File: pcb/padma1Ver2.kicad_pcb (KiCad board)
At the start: 2 copper layers, 33 x 68.6 mm, 15 parts, among them SW1 SPST

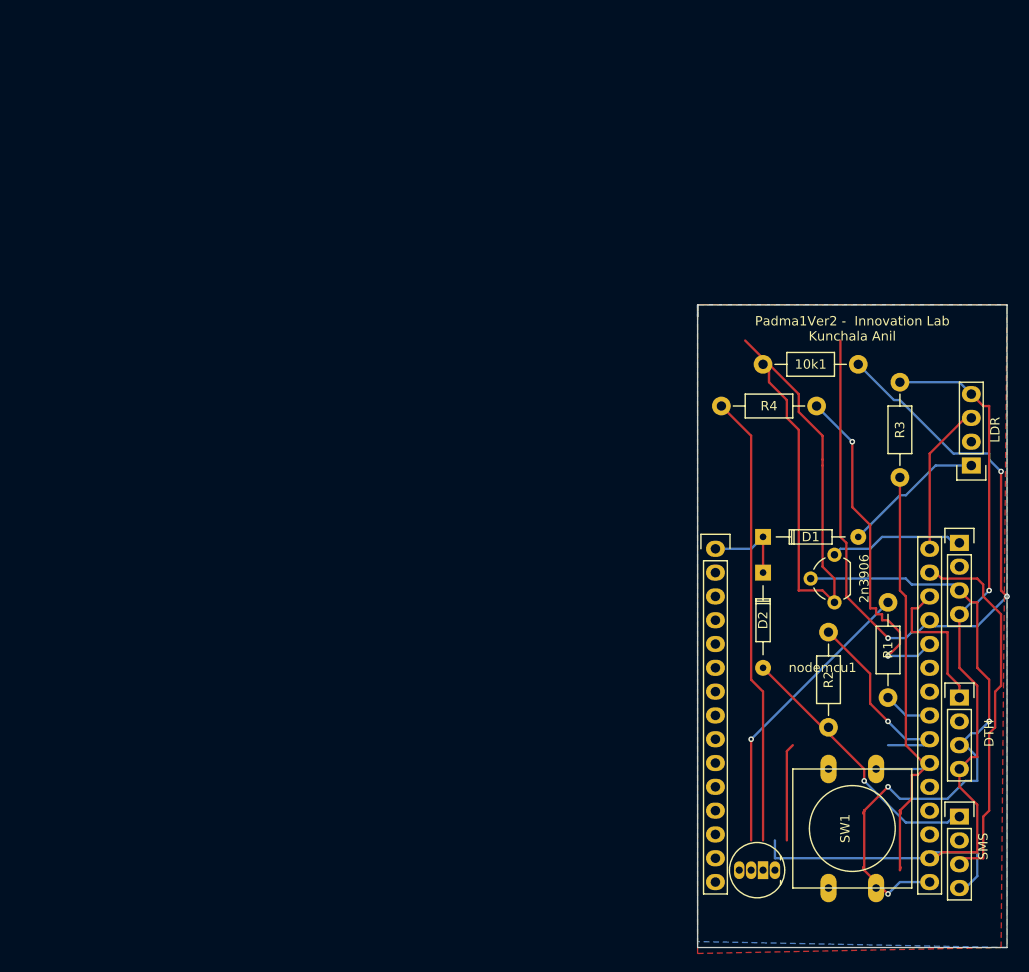
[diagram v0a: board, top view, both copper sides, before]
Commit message: pcb Without Any Errors
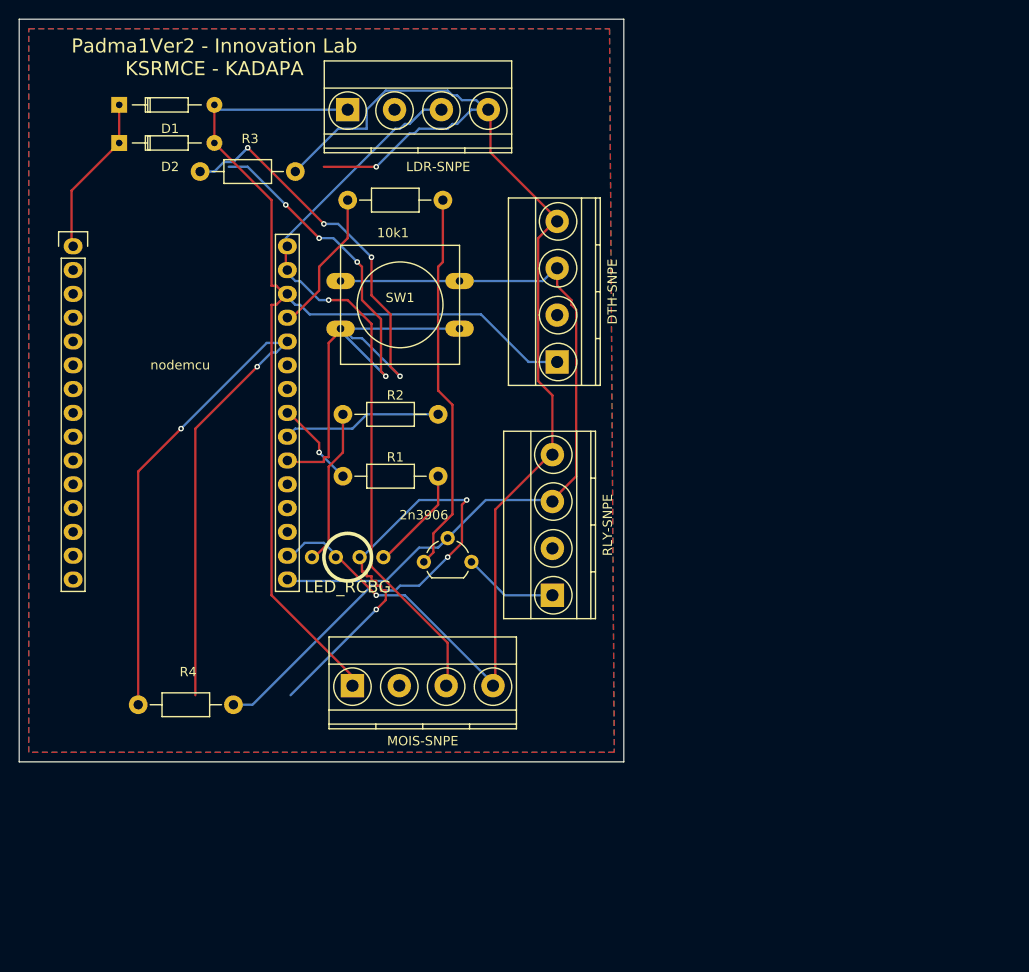
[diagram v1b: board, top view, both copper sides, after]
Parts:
- removed DTH, LDR, SMS: CONN_01X04, Pin_Headers:Pin_Header_Straight_1x04
- removed Grovr1: RLY, Pin_Headers:Pin_Header_Straight_1x04
- removed nodemcu1: nodemcu, nodemcu:NodeMCU_Amica_R2
- added DTH-SNPE: CONN_01X04, Terminal_Blocks:TerminalBlock_Pheonix_MKDS1.5-4pol, F.Cu at (128.5, 87.4)
- added LDR-SNPE: CONN_01X04, Terminal_Blocks:TerminalBlock_Pheonix_MKDS1.5-4pol, F.Cu at (106.2, 60.5)
- added MOIS-SNPE: CONN_01X04, Terminal_Blocks:TerminalBlock_Pheonix_MKDS1.5-4pol, F.Cu at (106.7, 121.9)
- added RLY-SNPE: RLY, Terminal_Blocks:TerminalBlock_Pheonix_MKDS1.5-4pol, F.Cu at (128.0, 112.3)
- added nodemcu: nodemcu, nodemcu:NodeMCU_Amica_R2, F.Cu at (76.9, 75.0)
- D3: value LED_RGB -> LED_RCBG; footprint LEDs:LED-RGB-5MM_Common_Cathode -> LED5_RGB:LED5_RGB_long_wide
- moved D1 82.7 mm to (81.8, 59.9)
- moved D2 82.6 mm to (81.8, 64.0), turned to 0 degrees
- moved R3 81.5 mm to (90.4, 67.1), turned to 0 degrees
- moved R4 79.1 mm to (83.8, 124.0), turned to 0 degrees
- moved SW1 73.8 mm to (111.8, 81.3), turned to 0 degrees
- moved R1 62.8 mm to (105.7, 99.6), turned to 0 degrees
- moved R2 61.6 mm to (105.7, 93.0), turned to 0 degrees
- moved D3 56.5 mm to (106.2, 108.2), turned to 0 degrees
- moved 2n3906 44.0 mm to (114.3, 108.7), turned to 0 degrees
- moved 10k1 38.4 mm to (116.3, 70.1), turned to 180 degrees
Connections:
- D1 pad 2: Net-(D1-Pad2) -> /signal
- D2 pad 2: Net-(D2-Pad2) -> /signal
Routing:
- net /signal: track 0.00 -> 117.0 mm
- net /power: track 0.00 -> 80.3 mm, vias 0 -> 1
- net Net-(10k1-Pad2): track 82.9 -> 16.0 mm, vias 3 -> 0
- net Net-(R3-Pad1): track 52.2 -> 117.8 mm, vias 0 -> 8
- net Net-(R4-Pad1): track 37.0 -> 88.7 mm
- net Earth: track 96.7 -> 146.4 mm, vias 1 -> 2
- net Net-(MOIS1-Pad3): track 39.8 -> 0.00 mm
- net Net-(D2-Pad2): track 28.8 -> 0.00 mm, vias 1 -> 0
- net Net-(D3-Pad3): track 48.2 -> 72.7 mm, vias 0 -> 3
- net Net-(10k1-Pad1): track 61.9 -> 40.7 mm
- net Net-(D3-Pad4): track 31.4 -> 11.2 mm, vias 1 -> 0
- net Net-(D3-Pad1): track 0.00 -> 16.8 mm
- net Net-(DTH1-Pad1): track 16.3 -> 0.00 mm
- net Net-(LDR1-Pad3): track 16.2 -> 0.00 mm
- net Net-(D1-Pad2): track 15.2 -> 0.00 mm
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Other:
- board size 33 x 68.6 mm -> 64.5 x 79.2 mm
- board text added: "Padma1Ver2 - Innovation Lab KSRMCE - KADAPA"
- board text removed: "Padma1Ver2 - Innovation Lab Kunchala Anil"
